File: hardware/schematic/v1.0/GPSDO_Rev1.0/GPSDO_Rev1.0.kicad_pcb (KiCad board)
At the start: 2 copper layers, 77.7 x 81.9 mm, 157 parts, among them CN1 LAIL-PHC2_54-2P-01-XH-L, J1 Conn_Coaxial, J3 Conn_01x04_Socket, J4 Conn_Coaxial, U1 TDC7200PWR, U10 SN74LVC1T45DBVR, U11 CH340E, U13 ISL55110IRZ-T, U14 TPS7A5201RPSR, U15 STM32G431CBU6, U16 TPS7A5201RPSR, U18 TPS2116DRLR, U2 LMK1C1103PWR, U3 TMP117AIDRVR, U4 TPS61023DRLR, U5 OCXO_20x20mm, U6 NEO-M8T-0, U7 OCXO_25.4x25.4mm, U8 REF5040, U9 OPA388IDR

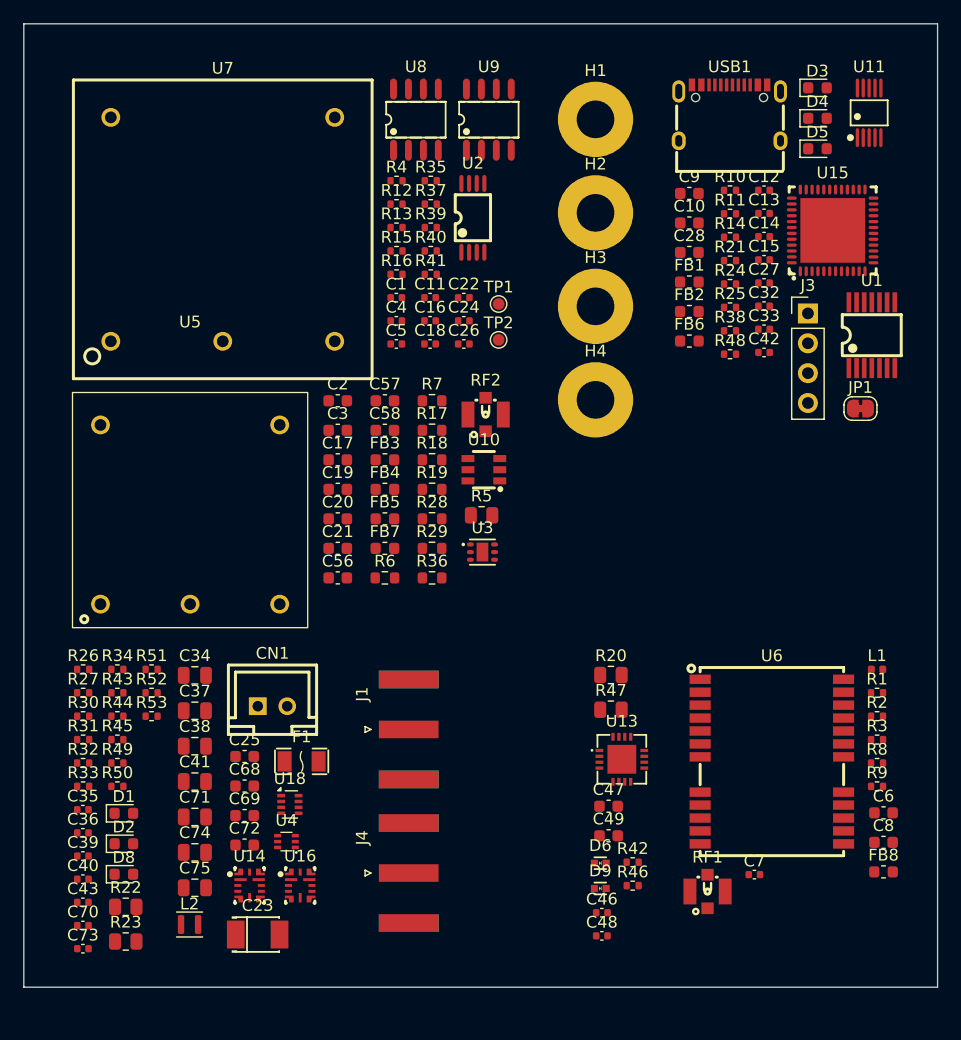
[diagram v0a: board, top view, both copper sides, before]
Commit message: sch and pcb update
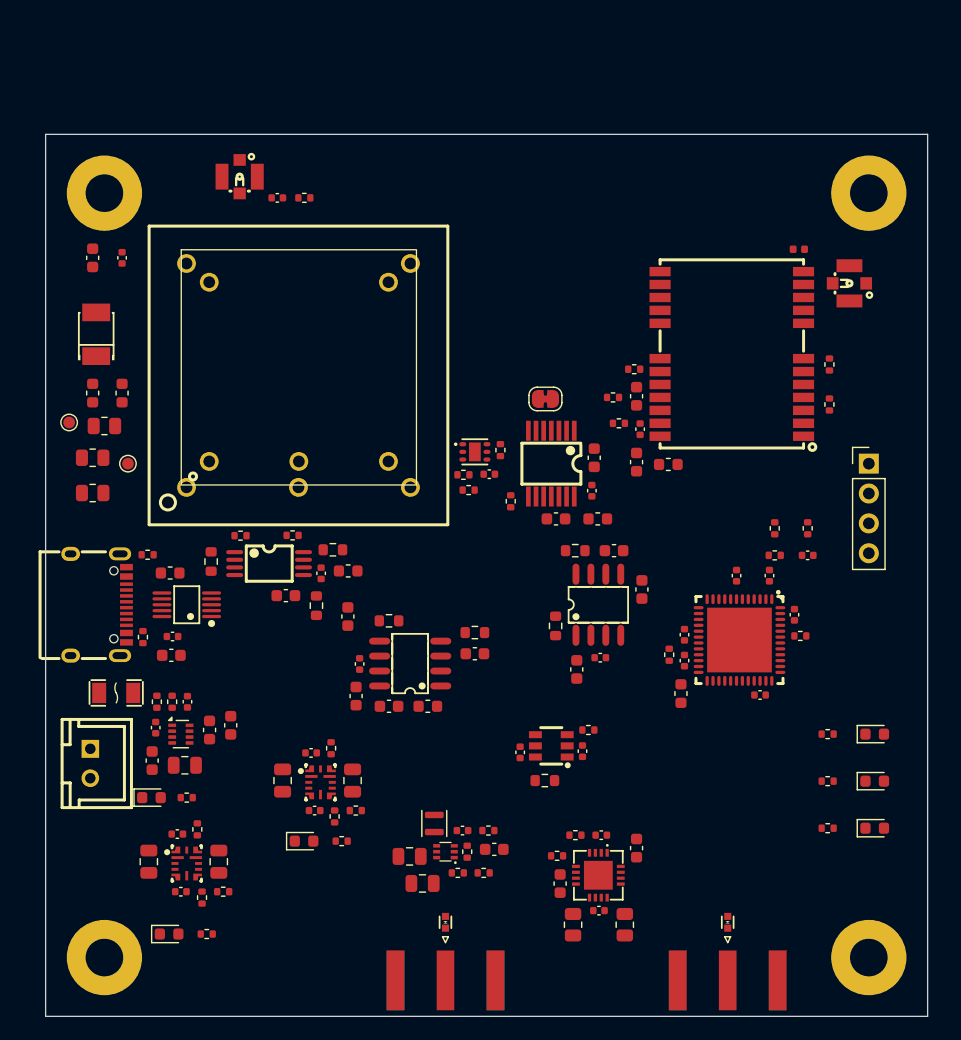
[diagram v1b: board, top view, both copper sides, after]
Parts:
- moved U11 71.5 mm to (118.4, 103.4), turned to 90 degrees
- moved H3 69.4 mm to (111.4, 133.4)
- moved USB1 68.0 mm to (110.9, 103.4), turned to -90 degrees
- moved R14 60.4 mm to (114.7, 106.2), turned to 90 degrees
- moved C27 58.6 mm to (117.2, 106.1)
- moved D5 58.0 mm to (176.9, 122.4)
- moved R11 57.4 mm to (115.1, 99.2), turned to 180 degrees
- moved D4 56.6 mm to (176.9, 118.4)
- moved C28 55.8 mm to (117.1, 107.7)
- moved D3 55.2 mm to (176.9, 114.4)
- moved RF1 53.1 mm to (174.8, 76.1), turned to 90 degrees
- moved C23 52.9 mm to (110.7, 80.4), turned to 90 degrees
- moved H4 52.8 mm to (176.4, 133.4)
- moved R35 48.6 mm to (152.6, 114.1)
- moved FB6 48.4 mm to (117.0, 100.7)
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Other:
- board size 77.7 x 81.9 mm -> 75 x 75 mm
- copper layers 2 -> 4
